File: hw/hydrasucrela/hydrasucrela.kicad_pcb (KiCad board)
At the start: 4 copper layers, 100 x 100 mm, 23 parts, among them J1 Conn_02x20_Odd_Even, J2 Conn_02x05_Odd_Even, J3 Conn_02x05_Odd_Even, J4 Conn_01x05, Q1 MMBTA06, U1 ECP5U_25_CABGA381, U3 TLV62569DRL, U4 NCP115CMX250TCG, U5 XUY73, U6 MCP23S08-E/SO

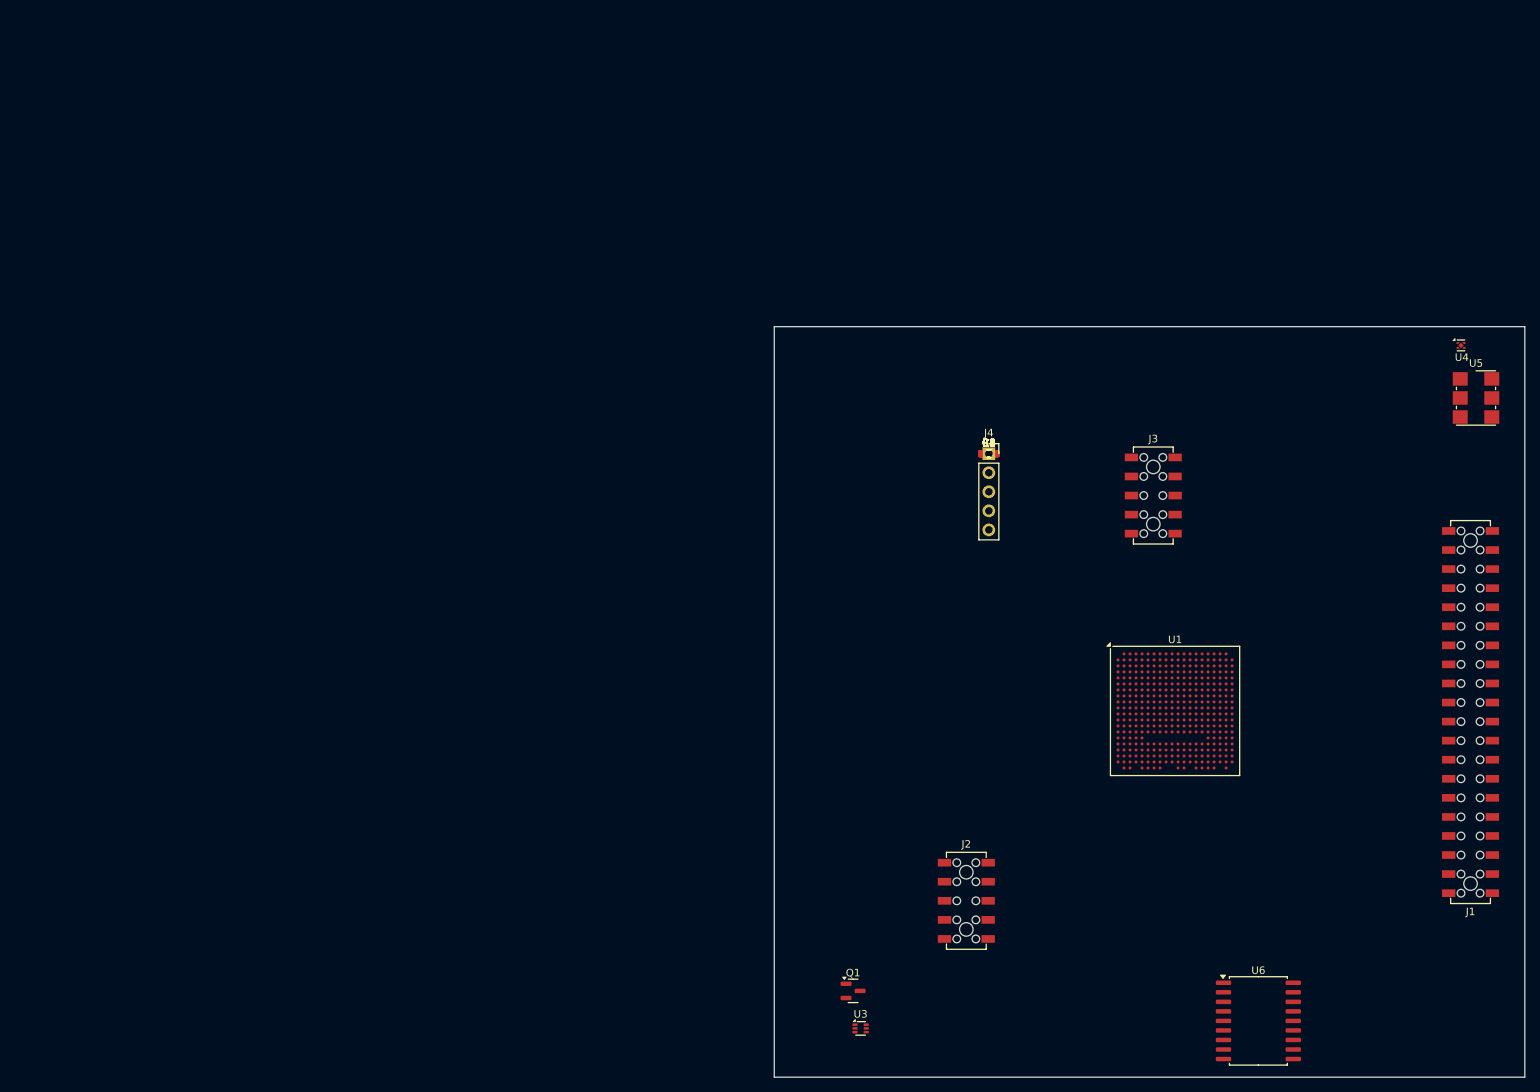
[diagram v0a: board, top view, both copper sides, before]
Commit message: Update HydraSucreLA PCB
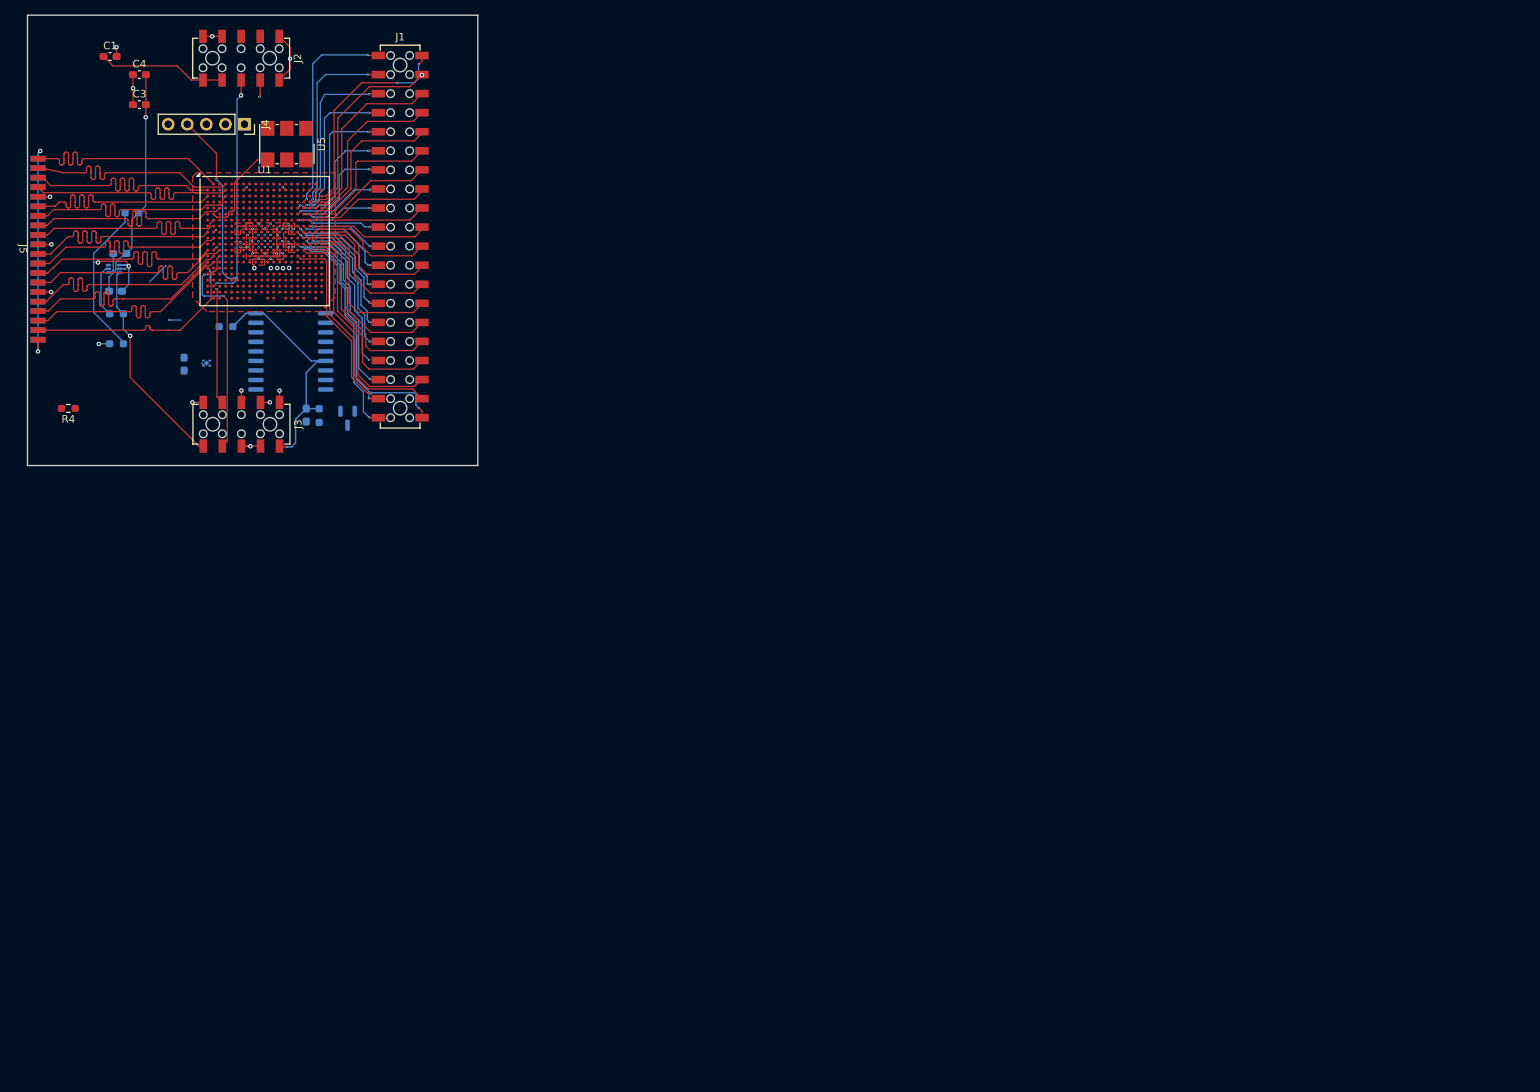
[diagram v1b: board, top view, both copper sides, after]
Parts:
- added J5: Conn_02x20_Top_Bottom, Library:probe_connector, F.Cu at (11.9, 43.1)
- C2, C5, C6, L1, Q1, R1, R2, R3, R5, R6, U3, U4, U6: moved to B.Cu
- moved U4 167.2 mm to (36.9, 58.4), turned to 180 degrees
- moved U5 162.0 mm to (47.5, 29.2), turned to -90 degrees
- moved U6 156.8 mm to (48.1, 56.8), turned to 180 degrees
- moved J1 156.1 mm to (62.6, 41.5), turned to 0 degrees
- moved J2 148.1 mm to (41.5, 17.7), turned to -90 degrees
- moved U3 141.9 mm to (24.5, 45.8), turned to 180 degrees
- moved U1 136.5 mm to (44.6, 42.1)
- moved C1 128.5 mm to (24.0, 17.5)
- moved C4 123.9 mm to (27.9, 19.9)
- moved R4 122.8 mm to (18.4, 64.4), turned to 180 degrees
- moved C3 122.4 mm to (27.9, 23.9)
- moved J3 121.9 mm to (41.5, 66.5), turned to -90 degrees
- moved L1 118.8 mm to (25.3, 43.8)
- moved R2 118.6 mm to (26.9, 38.3), turned to 180 degrees
- moved C2 118.4 mm to (24.7, 48.8), turned to 180 degrees
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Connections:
- J1 pad 10: HD23 -> HD12
- J1 pad 11: HD20 -> HD10
- J1 pad 12: HD21 -> HD8
- J1 pad 13: HD18 -> HD6
- J1 pad 14: HD19 -> HD4
- J1 pad 15: HD16 -> HD2
- J1 pad 16: HD17 -> HD0
- J1 pad 17: HD14 -> HTACK
- J1 pad 18: HD15 -> HRCLK
- J1 pad 19: HD12 -> HTRDY
- J1 pad 2: HD31 -> HD28
- J1 pad 20: HD13 -> HTCLK
- J1 pad 21: HD10 -> HD31
- J1 pad 22: HD11 -> HD29
- J1 pad 23: HD8 -> HD27
- J1 pad 24: HD9 -> HD25
- J1 pad 25: HD6 -> HD23
- J1 pad 26: HD7 -> HD21
- J1 pad 27: HD4 -> HD19
- J1 pad 28: HD5 -> HD17
- J1 pad 29: HD2 -> HD15
- J1 pad 3: HD28 -> HD26
- J1 pad 30: HD3 -> HD13
- J1 pad 31: HD0 -> HD11
- J1 pad 32: HD1 -> HD9
- J1 pad 33: HTACK -> HD7
- J1 pad 34: HRVLD -> HD5
- J1 pad 35: HRCLK -> HD3
- J1 pad 36: HRACT -> HD1
- J1 pad 37: HTRDY -> HRVLD
- J1 pad 38: HTVLD -> HRACT
- J1 pad 39: HTCLK -> HTVLD
- J1 pad 4: HD29 -> HD24
- J1 pad 5: HD26 -> HD22
- J1 pad 6: HD27 -> HD20
- J1 pad 7: HD24 -> HD18
- J1 pad 8: HD25 -> HD16
- J1 pad 9: HD22 -> HD14
- J2 pad 2: GND -> SCS0
- J2 pad 3: SCS0 -> MOSI0
- J2 pad 4: SCK0 -> GND
- J2 pad 5: MOSI0 -> GND
- J2 pad 6: MISO0 -> GND
- J2 pad 7: GND -> SCK0
- J2 pad 8: P5.0V -> MISO0
- J2 pad 9: GND -> P5.0V
- J3 pad 2: 3V3_IN -> GND
- J3 pad 4: GND -> RXD_1
- J3 pad 6: GND -> 3V3_IN
- J3 pad 7: RXD_1 -> GND
- J3 pad 8: TXD_1 -> GND
- J3 pad 9: GND -> TXD_1
- U1 pad A2: Probe_8 -> Probe_0
- U1 pad A4: Probe_0 -> Probe_1
- U1 pad A5: Probe_1 -> unconnected-(U1G-PL2B/-/HS/LDQ8-PadA5)
- U1 pad B1: Probe_9 -> Probe_2
- U1 pad C1: Probe_10 -> Probe_4
- U1 pad C18: HD0 -> unconnected-(U1D-PR2A/+/HS/RDQ8-PadC18)
- U1 pad C20: HD16 -> HD31
- U1 pad C4: Probe_2 -> Probe_5
- U1 pad D1: Probe_11 -> unconnected-(U1G-PL17B/-/HS/LDQ20-PadD1)
- U1 pad D17: HD1 -> HD30
- U1 pad D18: HD4 -> HD28
- U1 pad D19: HD17 -> HD29
- U1 pad D20: HD18 -> HD27
- U1 pad D5: Probe_5 -> unconnected-(U1G-PL8B/-/HS/LDQSN8-PadD5)
- U1 pad E16: HD2 -> HD22
- U1 pad E17: HD5 -> HD26
- U1 pad E18: HD6 -> HD24
- U1 pad E19: HD19 -> HD25
- U1 pad E20: HD20 -> HD23
- U1 pad E3: Probe_7 -> Probe_6
- U1 pad E4: Probe_4 -> unconnected-(U1G-PL8A/+/HS/LDQS8-PadE4)
- U1 pad F1: Probe_1 -> unconnected-(U1F-PL26B/-/PCLKC6_1/HS/LDQ32-PadF1)
- U1 pad F16: HD3 -> HD20
- U1 pad F17: HD8 -> HD18
- U1 pad F18: HD7 -> HD16
- U1 pad F20: HD22 -> HD19
- U1 pad F3: Probe_15 -> unconnected-(U1G-PL23B/-/PCLKC7_1/HS/LDQ20-PadF3)
- U1 pad F4: Probe_6 -> unconnected-(U1G-PL11A/+/HS/LDQ8-PadF4)
- U1 pad G16: HD10 -> HD14
- U1 pad G18: HD9 -> HD12
- U1 pad G19: HD24 -> HD17
- U1 pad G2: Probe_0 -> Probe_7
- U1 pad G20: HD23 -> HD15
- U1 pad G3: Probe_14 -> unconnected-(U1G-PL23A/+/PCLKT7_1/HS/LDQ20-PadG3)
- U1 pad G5: Probe_13 -> unconnected-(U1G-PL20B/-/HS/LDQSN20-PadG5)
- U1 pad H16: HD11 -> HD6
- U1 pad H17: HD13 -> HD8
- U1 pad H18: HD12 -> HD10
- U1 pad H20: HD25 -> HD13
- U1 pad H4: Probe_12 -> unconnected-(U1G-PL20A/+/GR_PCLK7_1/HS/LDQS20-PadH4)
- U1 pad J1: Probe_5 -> Probe_8
- U1 pad J16: HD15 -> HD2
- U1 pad J17: HD14 -> HD4
- U1 pad J18: HD26 -> HD0
- U1 pad J19: HD28 -> HD11
- U1 pad J20: HD30 -> HD9
- U1 pad J4: Probe_2 -> unconnected-(U1F-PL29A/+/GR_PCLK6_0/HS/LDQ32-PadJ4)
- U1 pad J5: Probe_3 -> unconnected-(U1F-PL29B/-/HS/LDQ32-PadJ5)
- U1 pad K18: HD27 -> HTACK
- U1 pad K19: HD29 -> HD7
- U1 pad K2: Probe_4 -> Probe_9
- U1 pad K20: HD31 -> HD5
- U1 pad K4: Probe_6 -> unconnected-(U1F-PL35A/+/HS/LDQ32-PadK4)
- U1 pad K5: Probe_7 -> unconnected-(U1F-PL35B/-/VREF1_6/HS/LDQ32-PadK5)
- U1 pad L16: HTRDY -> HTCLK
- U1 pad L17: HRCLK -> HTRDY
- U1 pad L18: HRACT -> HRCLK
- U1 pad L19: HTREQ -> HD3
- U1 pad L20: HTACK -> HD1
- U1 pad M1: Probe_13 -> Probe_10
- U1 pad M17: TXD_1 -> HTVLD
- U1 pad M18: HRVLD -> unconnected-(U1E-PR29D/-/RDQ32-PadM18)
- U1 pad M19: HTVLD -> HRVLD
- U1 pad M20: HTCLK -> HRACT
- U1 pad M4: Probe_8 -> unconnected-(U1F-PL38A/+/HS/LDQ44-PadM4)
- U1 pad N16: RXD_1 -> HTREQ
- U1 pad N3: Probe_10 -> Probe_15
- U1 pad N5: Probe_9 -> unconnected-(U1F-PL38B/-/HS/LDQ44-PadN5)
- U1 pad P1: Probe_14 -> Probe_13
- U1 pad P2: Probe_15 -> Probe_14
- U1 pad R1: unconnected-(U1H-PB4A/+/D7/IO7-PadR1) -> RXD_1
- U1 pad T1: unconnected-(U1H-PB4B/-/D6/IO6-PadT1) -> TXD_1
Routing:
- net GND: track 0.00 -> 64.6 mm, vias 0 -> 35
- net P5.0V: track 0.00 -> 45.5 mm, vias 0 -> 1
- net 3V3_IN: track 0.00 -> 39.4 mm, vias 0 -> 9
- net P1.1V: track 0.00 -> 37.4 mm, vias 0 -> 19
- net HTREQ: track 0.00 -> 33.9 mm, vias 0 -> 2
- net Probe_5: track 0.00 -> 32.0 mm
- net Probe_15: track 0.00 -> 32.0 mm
- net Probe_1: track 0.00 -> 32.0 mm
- net Probe_2: track 0.00 -> 32.0 mm
- net Net-(U3-FB): track 0.00 -> 31.9 mm, vias 0 -> 2
- net Probe_3: track 0.00 -> 31.9 mm
- net Probe_14: track 0.00 -> 31.9 mm
- net Probe_12: track 0.00 -> 31.9 mm
- net Probe_6: track 0.00 -> 31.9 mm
- net Probe_13: track 0.00 -> 31.9 mm
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- added copper zone on F.Cu, net 3V3_IN
- added copper zone on F.Cu, net GND
- added copper zone on In1.Cu, net GND
- added copper zone on F.Cu, net P1.1V
- added copper zone on F.Cu, net P1.8V
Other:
- board size 100 x 100 mm -> 60 x 60 mm
